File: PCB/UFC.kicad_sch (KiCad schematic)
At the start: 75 parts

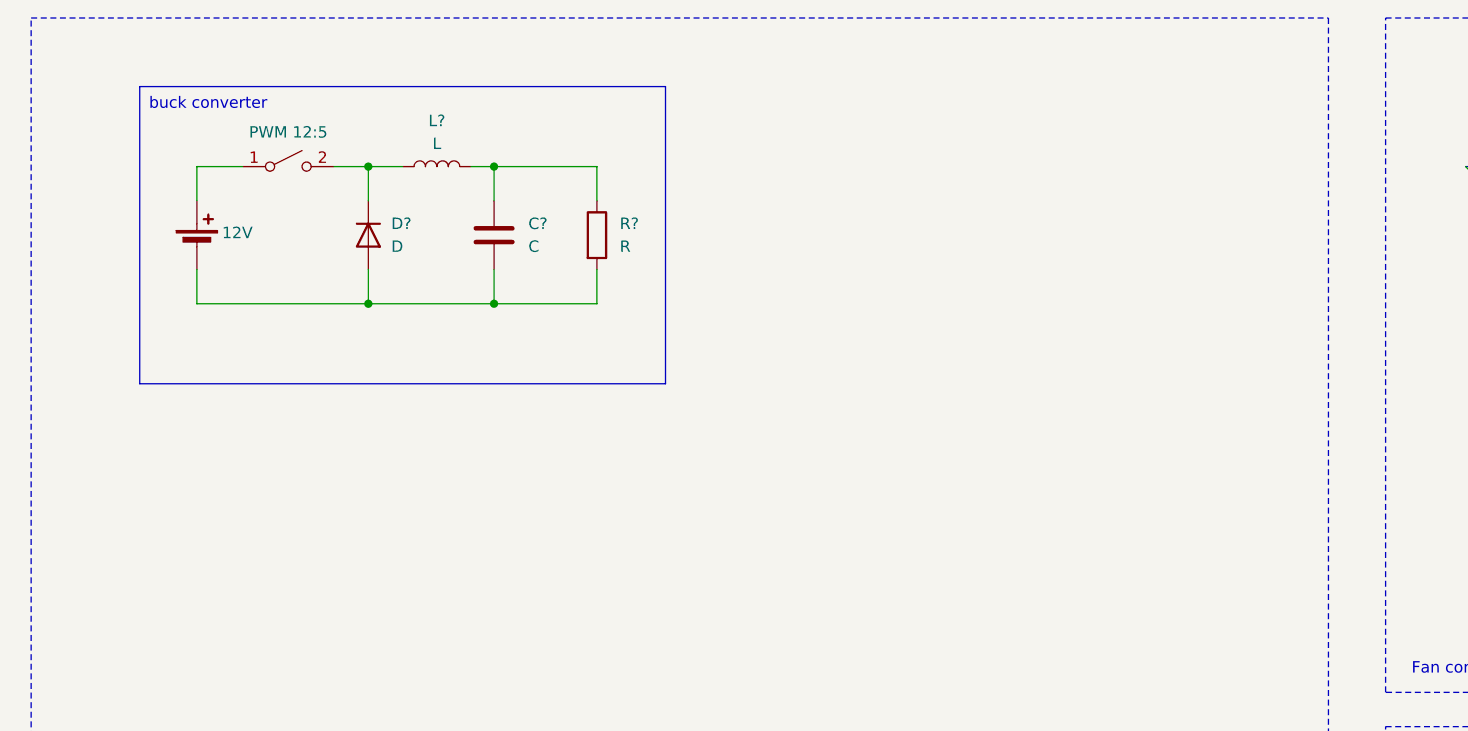
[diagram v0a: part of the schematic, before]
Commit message: tacho
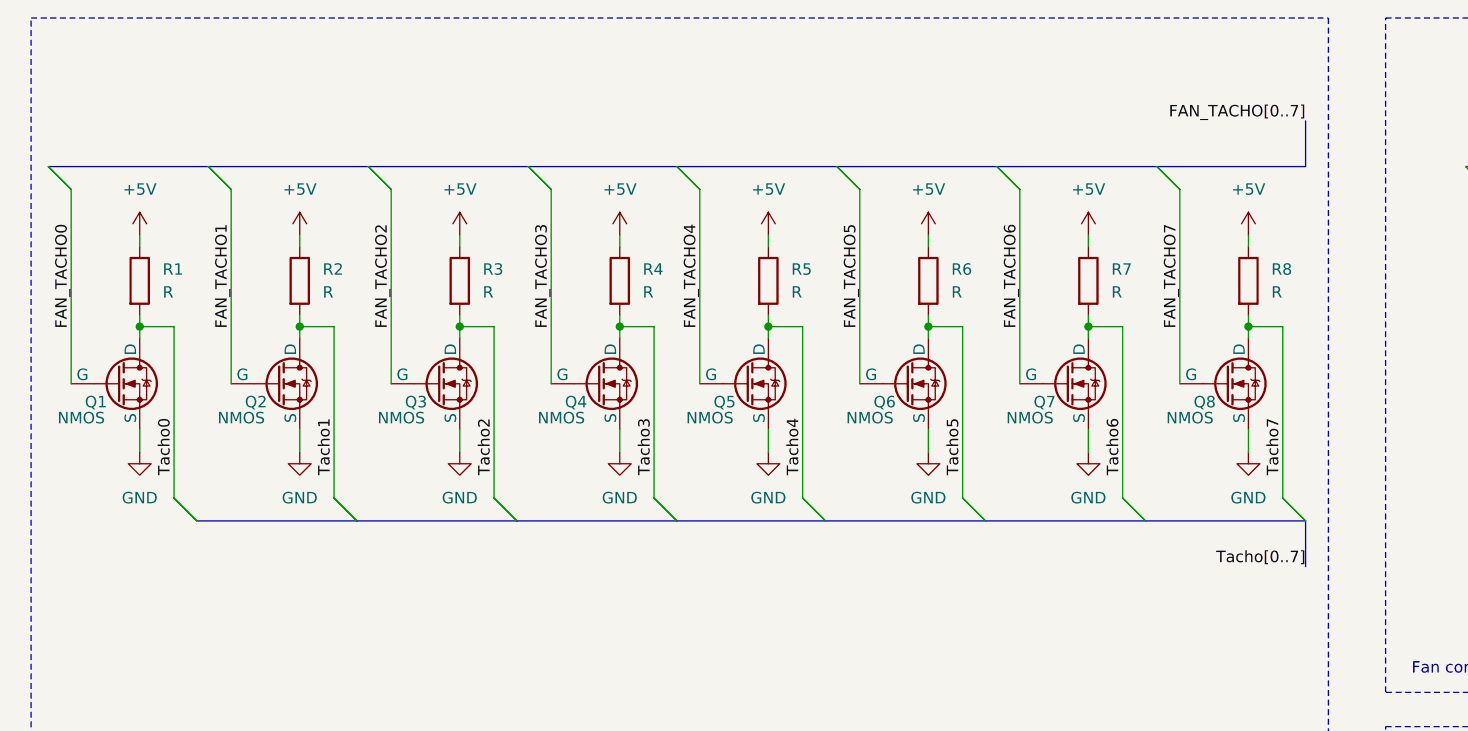
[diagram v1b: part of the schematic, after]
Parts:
- removed BT?: 12V, symbol Device:Battery_Cell
- removed C?: C, symbol Device:C
- removed D?: D, symbol Device:D
- removed L?: L, symbol Device:L
- removed R?: R, symbol Device:R
- removed SW?: PWM 12:5, symbol Switch:SW_SPST
- added Q1, Q2, Q3, Q4, Q5, Q6, Q7, Q8: NMOS, symbol Simulation_SPICE:NMOS
- added R1, R2, R3, R4, R5, R6, R7, R8: R, symbol Device:R
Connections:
- net +5V: now also R1.1, R2.1, R3.1, R4.1, R5.1, R6.1, R7.1, R8.1
- net FAN_TACHO0: now also Q1.2 (G)
- net FAN_TACHO1: now also Q2.2 (G)
- net FAN_TACHO2: now also Q3.2 (G)
- net FAN_TACHO3: now also Q4.2 (G)
- net FAN_TACHO4: now also Q5.2 (G)
- net FAN_TACHO5: now also Q6.2 (G)
- net FAN_TACHO6: now also Q7.2 (G)
- net FAN_TACHO7: now also Q8.2 (G)
- net GND: now also Q1.3 (S), Q2.3 (S), Q3.3 (S), Q4.3 (S), Q5.3 (S), Q6.3 (S), Q7.3 (S), Q8.3 (S)
- net Tacho0: now also Q1.1 (D), R1.2
- net Tacho1: now also Q2.1 (D), R2.2
- net Tacho2: now also Q3.1 (D), R3.2
- net Tacho3: now also Q4.1 (D), R4.2
- net Tacho4: now also Q5.1 (D), R5.2
- net Tacho6: now also Q7.1 (D), R7.2
- net Tacho7: now also Q8.1 (D), R8.2
- new net Tacho5: Q6.1 (D), R6.2
